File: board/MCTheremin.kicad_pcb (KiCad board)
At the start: 2 copper layers, 100 x 100 mm, 92 parts, among them J1 Barrel_Jack, J10 Conn_01x02, J11 Conn_01x01, J12 Conn_01x01, J13 Conn_01x01, J14 Conn_01x01, J15 Conn_01x01, J16 Conn_01x01, J17 Conn_01x02, J18 Conn_01x01, J19 Conn_01x04, J2 Conn_01x02, J20 Conn_01x04, J21 Conn_01x02, J22 Conn_01x02, J3 Conn_01x01, J4 Conn_01x01, J5 Conn_01x02, J6 Conn_01x02, J7 Conn_01x01, J8 Conn_01x01, J9 Conn_01x01, Q1 2N3904, Q2 2N3904, Q3 2N3904, SW1 SW_Push, SW2 SW_Push, U1 74HC04, U2 MCP4921, U3 LM7805_TO220, U4 LM386, U5 LM358, U6 74HC04

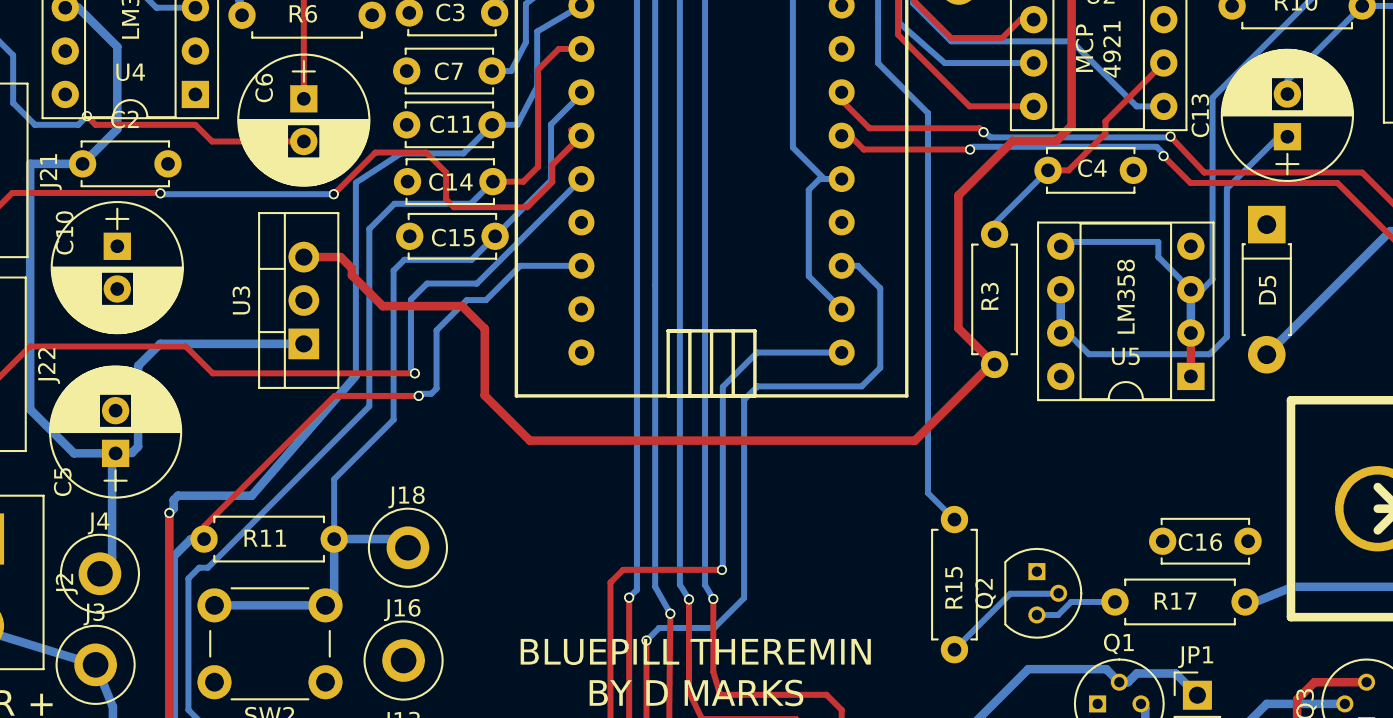
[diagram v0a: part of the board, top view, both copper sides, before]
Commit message: Pre LC
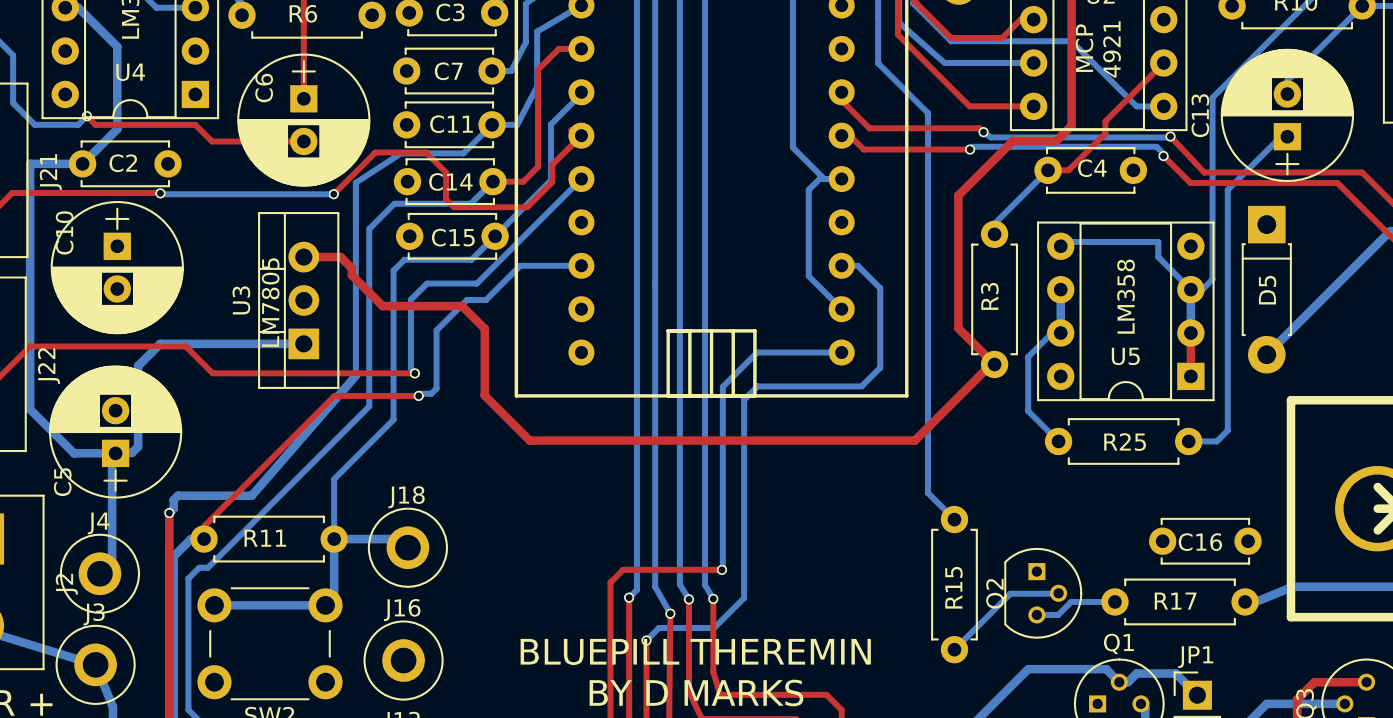
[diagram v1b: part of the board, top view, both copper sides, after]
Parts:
- added R25: 1k, Resistors_THT:R_Axial_DIN0207_L6.3mm_D2.5mm_P7.62mm_Horizontal, F.Cu at (120.9, 110.6)
- R10: value 10k -> 220R
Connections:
- U5 pad 6: Net-(C13-Pad1) -> Net-(R25-Pad1)
- U5 pad 7: Net-(C13-Pad1) -> Net-(R25-Pad1)
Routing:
- net Net-(R25-Pad1): track 0.00 -> 11.1 mm
- net Net-(C13-Pad1): track 26.7 -> 21.9 mm
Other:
- board text added: "LM7805"
